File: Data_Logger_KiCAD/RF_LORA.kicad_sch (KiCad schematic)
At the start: 16 parts, among them U6 SX1262IMLTRT, U7 MASW-007221

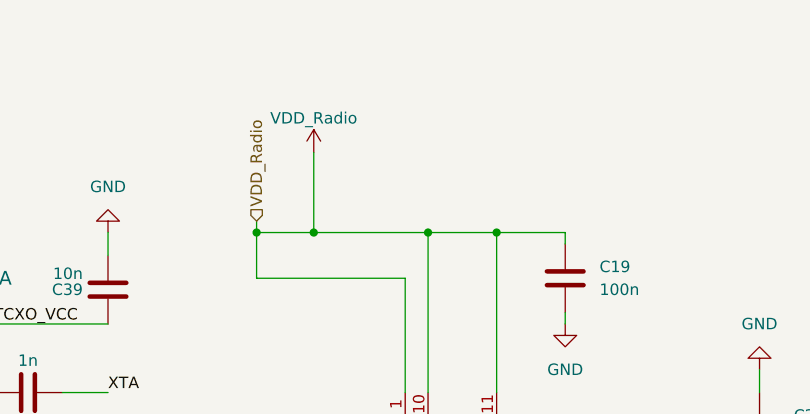
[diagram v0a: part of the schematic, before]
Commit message: save point
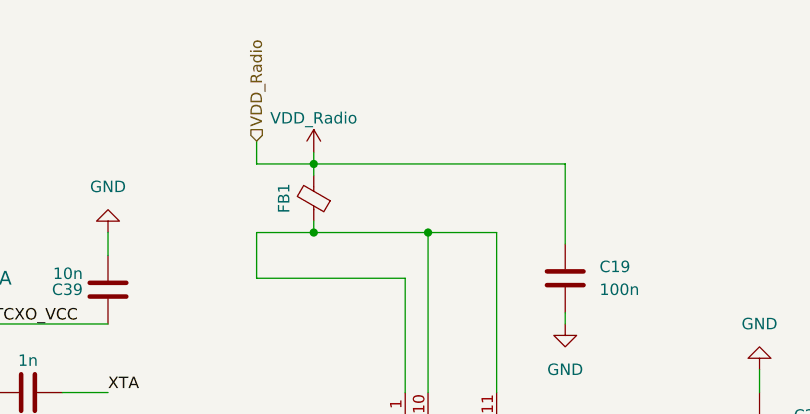
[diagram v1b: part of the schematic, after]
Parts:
- added FB1: FerriteBead_Small, Inductor_SMD:L_0603_1608Metric, symbol Device:FerriteBead_Small
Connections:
- net VDD_Radio: now also FB1.2; no longer U6.1 (VDD_IN), U6.10 (VBAT), U6.11 (VBAT_IO)
- new net: FB1.1, U6.1 (VDD_IN), U6.10 (VBAT), U6.11 (VBAT_IO)
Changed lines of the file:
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@@
 	(paper "A4")
+	(junction
+		(at 83.82 30.48)
+		(diameter 0)
+		(color 0 0 0 0)
+	)
 	(junction
 		(at 96.52 38.1)
@@
 	)
 	(junction
-		(at 104.14 38.1)
-		(diameter 0)
-		(color 0 0 0 0)
-	)
-	(junction
 		(at 203.2 113.03)
-		(diameter 0)
-		(color 0 0 0 0)
-	)
-	(junction
-		(at 77.47 38.1)
 		(diameter 0)
 		(color 0 0 0 0)
@@
 	(wire
 		(pts
-			(xy 83.82 29.21) (xy 83.82 38.1)
+			(xy 83.82 30.48) (xy 77.47 30.48)
+		)
+		(stroke
+			(width 0)
+			(type default)
+		)
+	)
+	(wire
+		(pts
+			(xy 83.82 29.21) (xy 83.82 30.48)
 		)
 		(stroke
@@
 	(wire
 		(pts
-			(xy 77.47 36.83) (xy 77.47 38.1)
-		)
-		(stroke
-			(width 0)
-			(type default)
-		)
-	)
-	(wire
-		(pts
 			(xy 62.23 101.6) (xy 83.82 101.6)
 		)
@@
 	(wire
 		(pts
+			(xy 77.47 27.94) (xy 77.47 30.48)
+		)
+		(stroke
+			(width 0)
+			(type default)
+		)
+	)
+	(wire
+		(pts
 			(xy 24.13 52.07) (xy 24.13 55.88)
 		)
@@
 	(wire
 		(pts
+			(xy 83.82 36.83) (xy 83.82 38.1)
+		)
+		(stroke
+			(width 0)
+			(type default)
+		)
+	)
+	(wire
+		(pts
 			(xy 130.81 63.5) (xy 133.35 63.5)
 		)
@@
 	(wire
 		(pts
-			(xy 104.14 38.1) (xy 111.76 38.1)
-		)
-		(stroke
-			(width 0)
-			(type default)
-		)
-	)
-	(wire
-		(pts
 			(xy 203.2 113.03) (xy 213.36 113.03)
 		)
@@
 	(wire
 		(pts
-			(xy 104.14 38.1) (xy 96.52 38.1)
-		)
-		(stroke
-			(width 0)
-			(type default)
-		)
-	)
-	(wire
-		(pts
 			(xy 120.65 69.85) (xy 120.65 71.12)
 		)
@@
 	(wire
 		(pts
-			(xy 96.52 38.1) (xy 83.82 38.1)
+			(xy 96.52 38.1) (xy 104.14 38.1)
 		)
 		(stroke
@@
 	(wire
 		(pts
+			(xy 111.76 30.48) (xy 111.76 39.37)
+		)
+		(stroke
+			(width 0)
+			(type default)
+		)
+	)
+	(wire
+		(pts
 			(xy 167.64 83.82) (xy 187.96 83.82)
 		)
@@
 	(wire
 		(pts
+			(xy 83.82 38.1) (xy 96.52 38.1)
+		)
+		(stroke
+			(width 0)
+			(type default)
+		)
+	)
+	(wire
+		(pts
 			(xy 120.65 69.85) (xy 132.08 69.85)
 		)
@@
 	(wire
 		(pts
-			(xy 111.76 38.1) (xy 111.76 39.37)
-		)
-		(stroke
-			(width 0)
-			(type default)
-		)
-	)
-	(wire
-		(pts
 			(xy 128.27 66.04) (xy 130.81 66.04)
 		)
@@
 		(pts
 			(xy 96.52 55.88) (xy 96.52 38.1)
+		)
+		(stroke
+			(width 0)
+			(type default)
+		)
+	)
+	(wire
+		(pts
+			(xy 83.82 30.48) (xy 111.76 30.48)
+		)
+		(stroke
+			(width 0)
+			(type default)
+		)
+	)
+	(wire
+		(pts
+			(xy 83.82 30.48) (xy 83.82 31.75)
 		)
 		(stroke
@@
 	(hierarchical_label "VDD_Radio"
 		(shape input)
-		(at 77.47 36.83 90)
+		(at 77.47 27.94 90)
 		(effects
 			(font
@@
 					(unit 1)
 				)
+			)
+		)
+	)
+	(symbol
+		(lib_id "Device:FerriteBead_Small")
+		(at 83.82 34.29 180)
+		(unit 1)
+		(exclude_from_sim no)
+		(in_bom yes)
+		(on_board yes)
+		(dnp no)
+		(property "Reference" "FB1"
+			(at 80.518 34.29 90)
+			(effects
+				(font
+					(size 1.27 1.27)
+				)
+			)
+		)
+		(property "Value" "FerriteBead_Small"
+			(at 80.01 34.3281 90)
+			(effects
+				(font
+					(size 1.27 1.27)
+				)
+				(hide yes)
+			)
+		)
+		(property "Footprint" "Inductor_SMD:L_0603_1608Metric"
+			(at 85.598 34.29 90)
+			(effects
+				(font
+					(size 1.27 1.27)
+				)
+				(hide yes)
+			)
+		)
+		(property "Datasheet" "~"
+			(at 83.82 34.29 0)
+			(effects
+				(font
+					(size 1.27 1.27)
+				)
+				(hide yes)
+			)
+		)
+		(property "Description" "Ferrite bead, small symbol"
+			(at 83.82 34.29 0)
+			(effects
+				(font
+					(size 1.27 1.27)
+				)
+				(hide yes)
+			)
+		)
+		(property "LCSC" " C14709"
+			(at 83.82 34.29 90)
+			(effects
+				(font
+					(size 1.27 1.27)
+				)
+				(hide yes)
+			)
+		)
+		(pin "2"
+		)
+		(pin "1"
+		)
+		(instances
+			(project "Data_Logger_Board"
+				(path "/db968e42-3ace-4cc9-9096-9d8f48135c40/795ab2be-9db7-4254-b05c-ac2b60177344/ddd17302-66df-4ba5-8c9c-bee0e050b0e0"
+					(reference "FB1")
+					(unit 1)
+				)
